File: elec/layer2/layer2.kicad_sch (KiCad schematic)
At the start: 47 parts, among them J1 Conn_01x03, J10 Conn_01x05, J11 Conn_01x05, J12 XT60-M, J17 Conn_01x02, J18 Conn_01x02, J2 XT30UPB-M, J3 Conn_01x04, J4 Conn_01x05, J5 Conn_01x03, J6 XT30PW-M, J7 XT30PW-M, J8 XT30PW-M, J9 XT30PW-M, SW1 SW_SPDT_312, U1 TEENSY40

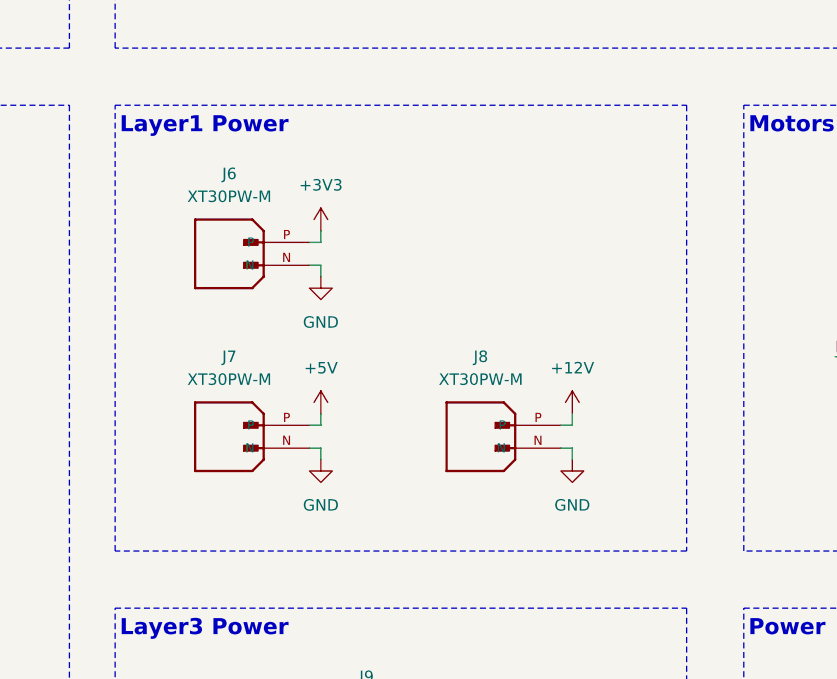
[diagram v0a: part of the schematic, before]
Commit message: chore: l2
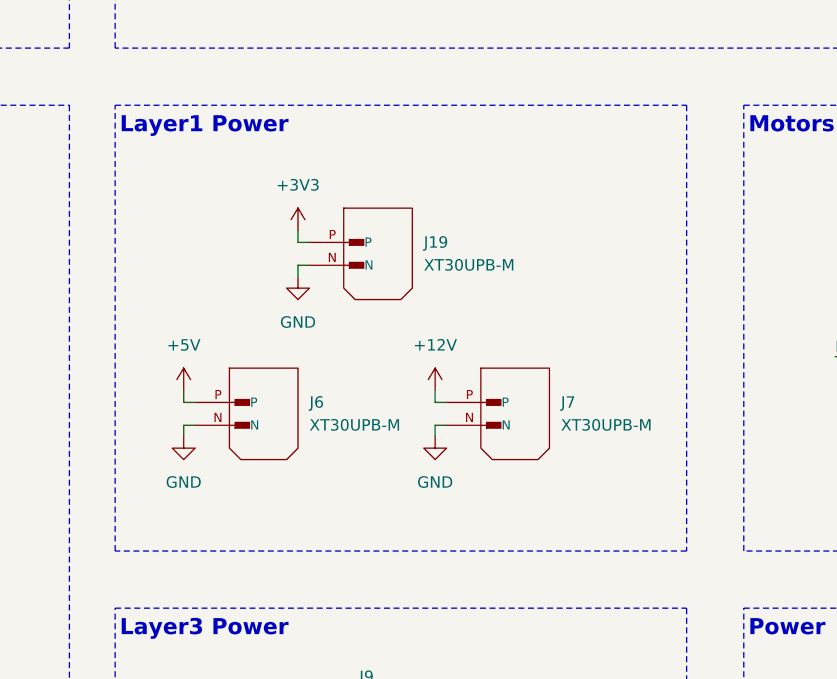
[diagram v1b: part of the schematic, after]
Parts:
- removed J6, J7, J8: XT30PW-M, layer2-pcb-footprints:AMASS_XT30PW-M, symbol layer1-pcb-symbols:XT30PW-M
- added J19, J6, J7: XT30UPB-M, layer2-pcb-footprints:AMASS_XT30UPB-M, symbol layer2-pcb-symbols:XT30UPB-M
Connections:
- net +12V: now also J7.P
- net +3V3: now also J19.P
- net +5V: now also J6.P
- net GND: now also J19.N, J6.N, J7.N
